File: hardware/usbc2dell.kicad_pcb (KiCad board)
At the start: 2 copper layers, 39.5 x 26.5 mm, 28 parts, among them J1 USB_C_Receptacle_PowerOnly_6P, J2 DELL_Charger, Q1 Q_NMOS_GDS, Q2 Q_NPN_BEC, SW1 SW_DIP_x04, U1 ATtiny1616-M, U2 FUSB302BMPX, U3 L7805

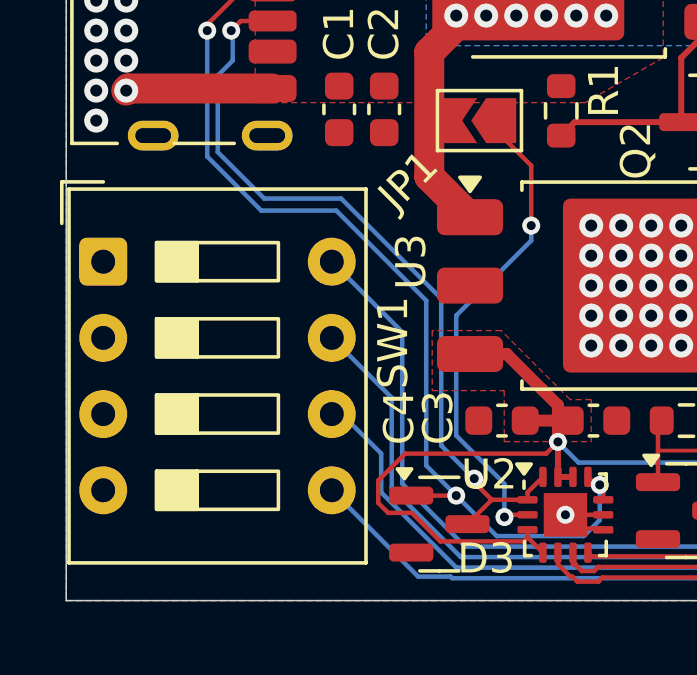
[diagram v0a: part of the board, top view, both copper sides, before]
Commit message: DRC
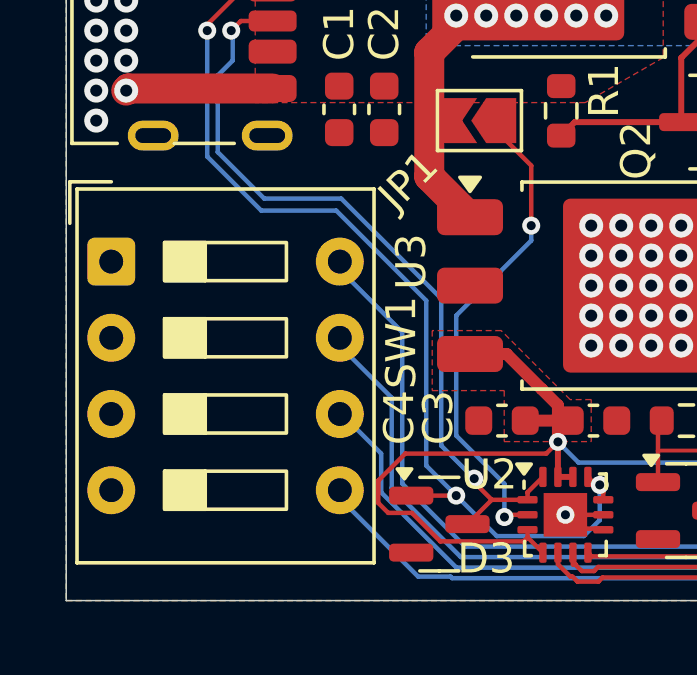
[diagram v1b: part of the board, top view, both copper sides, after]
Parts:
- moved SW1 0.27 mm to (89.0, 73.2)
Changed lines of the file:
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@@
 			)
 		)
-		(attr board_only exclude_from_pos_files exclude_from_bom)
+		(attr board_only exclude_from_pos_files exclude_from_bom allow_missing_courtyard)
 		(fp_circle
 			(center 0 0)
@@
 			)
 		)
-		(attr board_only exclude_from_pos_files exclude_from_bom)
+		(attr board_only exclude_from_pos_files exclude_from_bom allow_missing_courtyard)
 		(fp_circle
 			(center 0 0)
@@
 	(footprint "Button_Switch_THT:SW_DIP_SPSTx04_Slide_9.78x12.34mm_W7.62mm_P2.54mm"
 		(layer "F.Cu")
-		(at 88.7325 73.2025)
+		(at 89 73.2)
 		(descr "4x-dip-switch SPST , Slide, row spacing 7.62 mm (300 mils), body size 9.78x12.34mm (see e.g. https://www.ctscorp.com/wp-content/uploads/206-208.pdf)")
 		(tags "DIP Switch SPST Slide 7.62mm 300mil")
@@
 		(sheetname "/")
 		(sheetfile "usbc2dell.kicad_sch")
-		(attr through_hole)
+		(attr through_hole allow_missing_courtyard)
 		(fp_line
 			(start 13.92 -5.12)
